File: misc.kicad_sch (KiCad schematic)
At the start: 64 parts, among them J16 Screw_Terminal_01x10, J17 Conn_Coaxial, J18 Conn_02x13_Odd_Even, J19 Conn_02x13_Odd_Even, M10 M3 Solder Nut, M6 Fan, M7 M3 Solder Nut, M8 M3 Solder Nut, M9 M3 Solder Nut, U10 TPP60508, U11 TPP60508

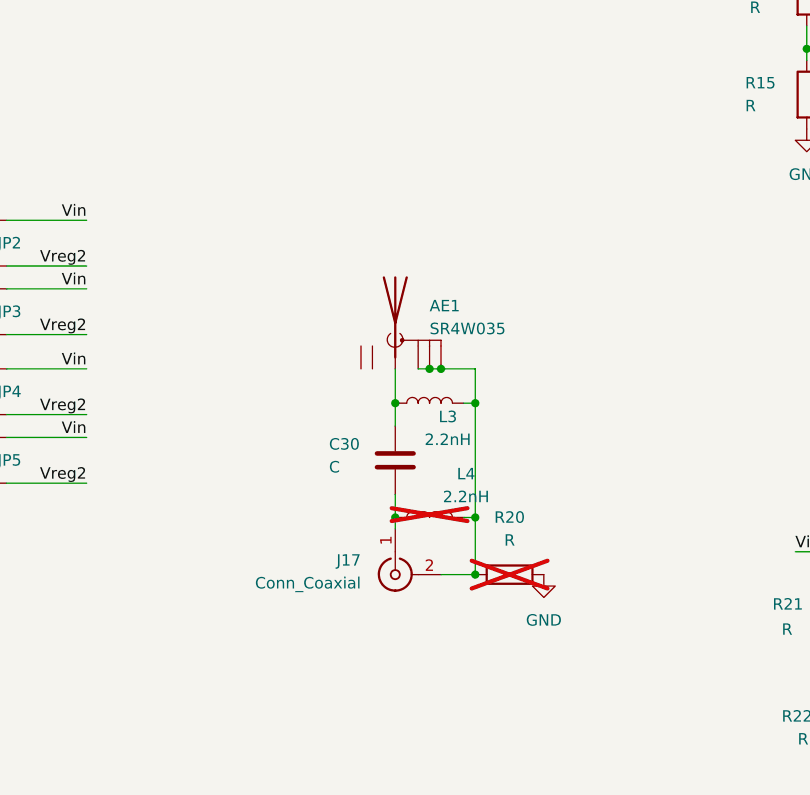
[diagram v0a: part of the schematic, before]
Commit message: pre-revise 5v route
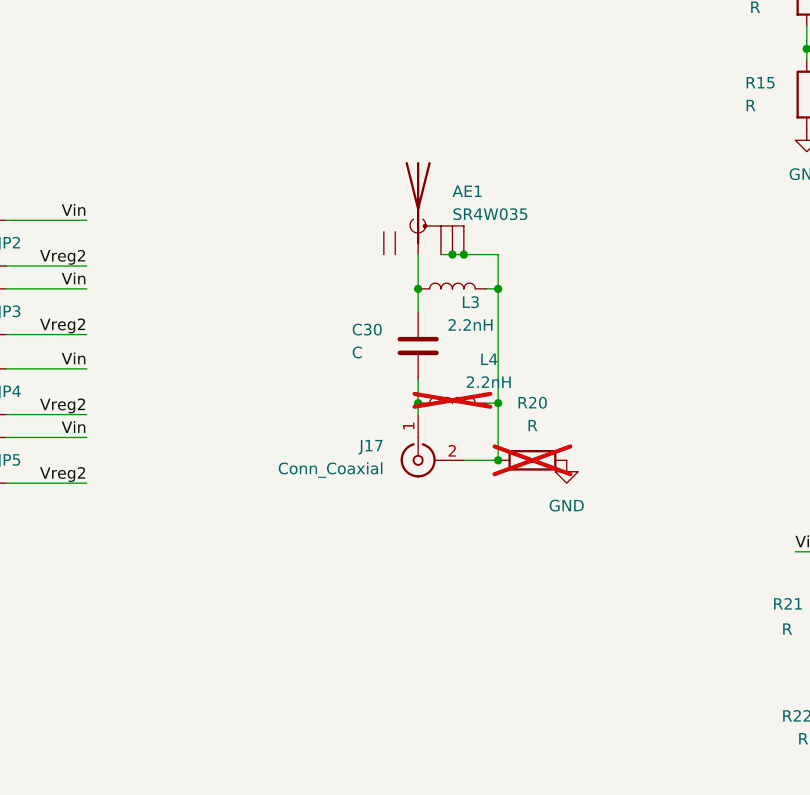
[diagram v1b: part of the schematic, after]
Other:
- moved on the sheet: AE1, C30, J17, L3, L4, R20
